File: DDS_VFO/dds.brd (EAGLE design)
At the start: 93.5 x 78.7 mm, 48 parts

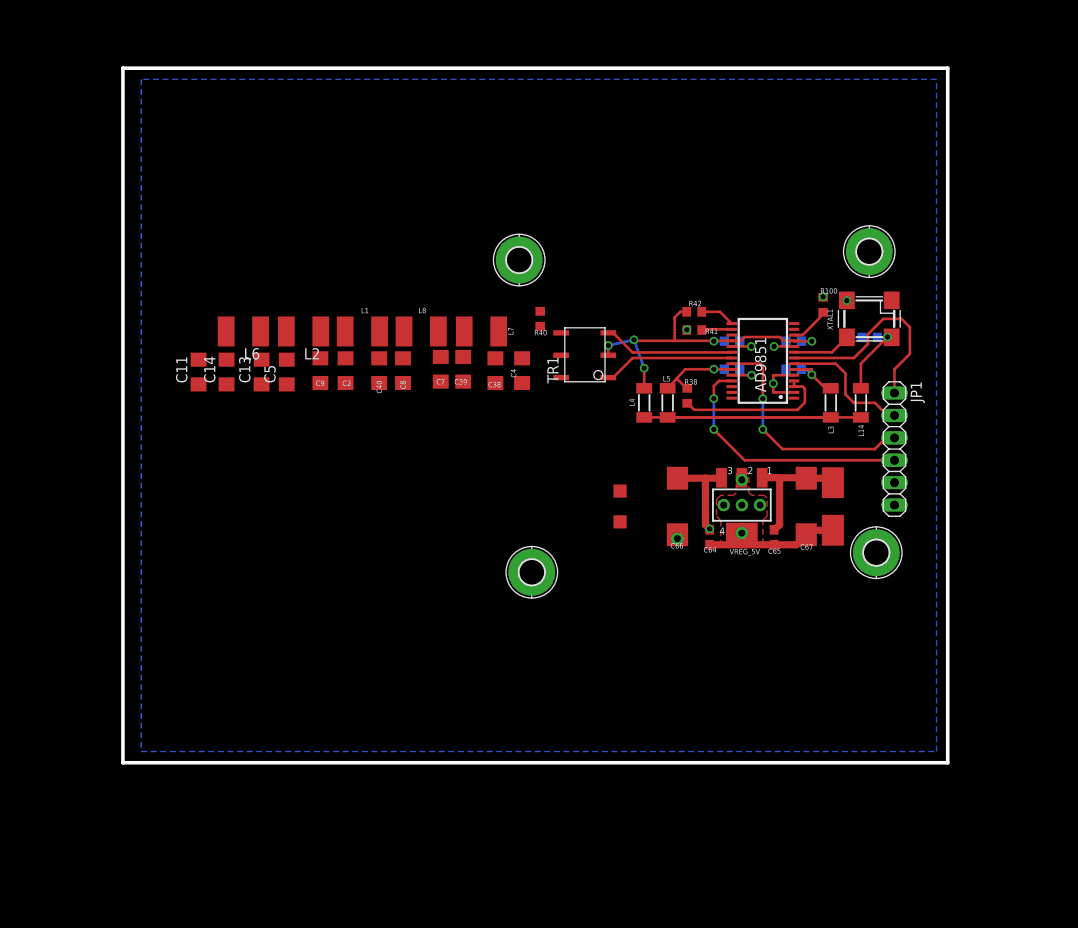
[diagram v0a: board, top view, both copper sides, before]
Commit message: Almost done.
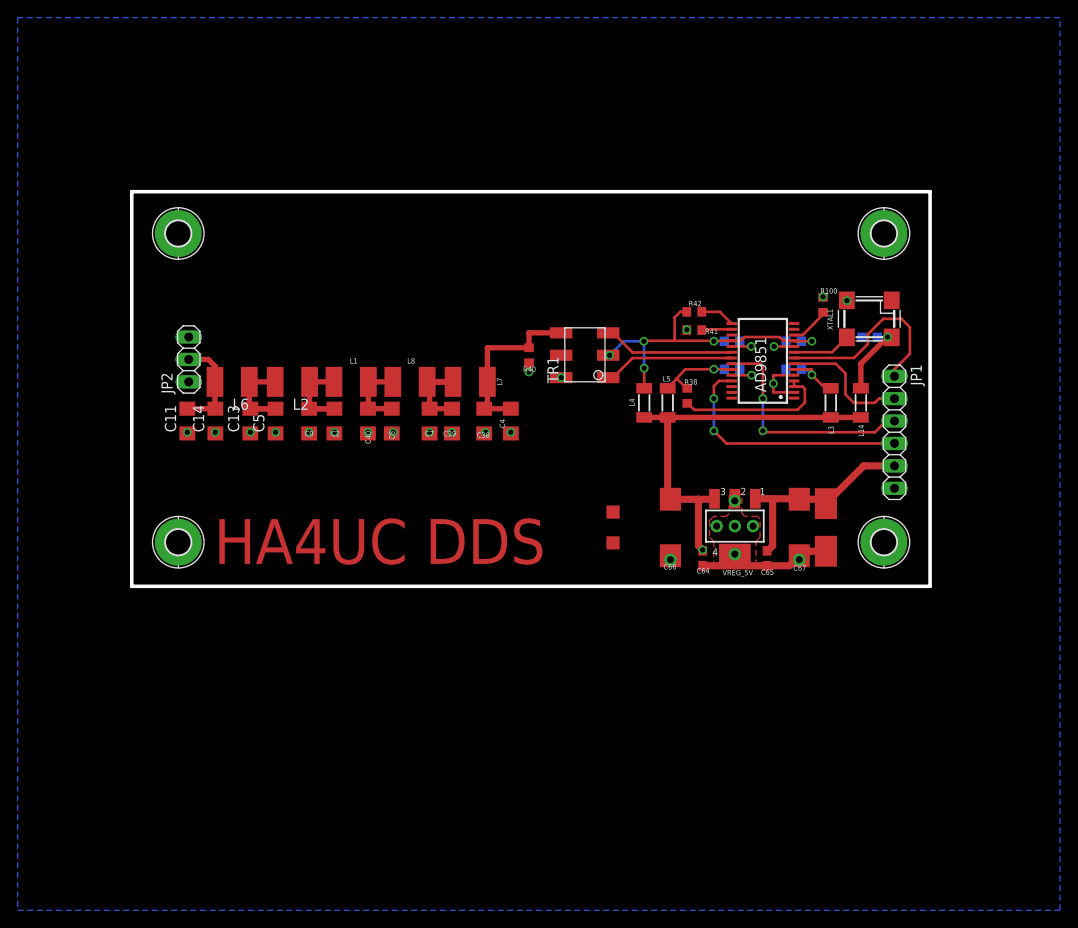
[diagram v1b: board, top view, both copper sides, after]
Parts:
- added JP2: (no value), pinhead:1X03
- moved H2 78.4 mm to (-25.0, 60.0)
- moved H4 52.3 mm to (55.0, 25.0)
- moved H3 40.2 mm to (-25.0, 25.0)
- moved H1 36.2 mm to (55.0, 60.0)
- moved C39 6.01 mm to (6.03, 38.7)
- moved C7 6.01 mm to (3.49, 38.7)
- moved C2 5.85 mm to (-7.30, 38.7)
- moved C38 5.85 mm to (9.68, 38.7)
- moved C4 5.85 mm to (12.7, 38.7)
- moved C40 5.85 mm to (-3.49, 38.7)
- moved C8 5.85 mm to (-0.79, 38.7)
- moved C9 5.85 mm to (-10.2, 38.7)
- moved L1 5.85 mm to (-5.40, 43.2)
- moved L2 5.85 mm to (-12.1, 43.2)
- moved L6 5.85 mm to (-18.9, 43.2)
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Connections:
- removed net BATT+: C65.1, C67.+, U$8.P$1, VREG_5V.1
- net FILTERED: now also JP2.2
- net GND: now also JP2.1, JP2.3
- net VCC: now also C65.1, C67.+, U$8.P$1, VREG_5V.1
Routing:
- net VCC: track 0.00 -> 24.1 mm
- net DDSOUT: track 0.00 -> 20.3 mm
- net BATT+: track 14.5 -> 0.00 mm
- net N$6: track 0.00 -> 11.8 mm
- net N$2: track 0.00 -> 11.5 mm
- net FILTERED: track 0.00 -> 11.3 mm
- net N$74: track 0.00 -> 11.2 mm
- net +5V: track 54.1 -> 45.1 mm
- net N$1: track 0.00 -> 8.56 mm
- net GND: track 31.1 -> 33.9 mm, vias 13 -> 28
- net DDS_FQ_UD: track 24.2 -> 22.3 mm
- net AVDD: track 37.1 -> 36.2 mm
- net DDS_RESET: track 27.2 -> 26.5 mm
- net DDS_DATA: track 29.1 -> 28.4 mm
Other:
- board size 93.5 x 78.7 mm -> 90.5 x 44.7 mm
- board text added: "HA4UC DDS"
